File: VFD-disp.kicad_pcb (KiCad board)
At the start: 2 copper layers, 120.2 x 65.5 mm, 97 parts, among them J1 USB_C_Receptacle_USB2.0_14P, J2 Conn_02x04_Odd_Even, J3 Jack-DC, J4 Conn_02x04_Odd_Even, J5 Conn_02x04_Odd_Even, J6 Conn_02x04_Odd_Even, Q1 NMOS, Q3 NMOS, SW1 SW_SPST, U1 ESP32-C6-WROOM-1, U10 TXS0104EPW, U11 MAX811TEUS-T, U12 MCP4728, U2 FUSB302B01MPX, U3 LM1117DT-3.3, U4 MCP1416, U5 LM2576HVS-ADJ, U6 MAX1771xSA, U7 LM2576HVS-ADJ, U9 FM24C64B, Y1 Crystal

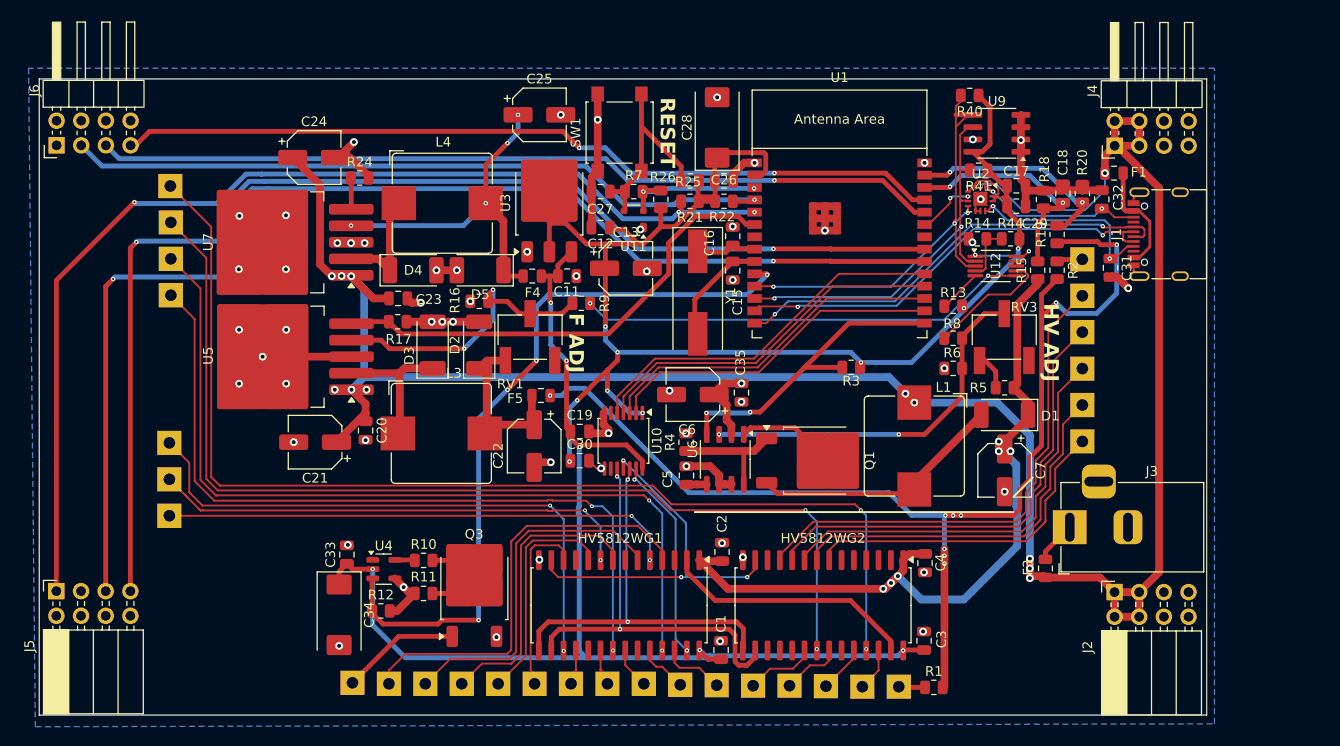
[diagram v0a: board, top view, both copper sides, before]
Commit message: We need to golf!
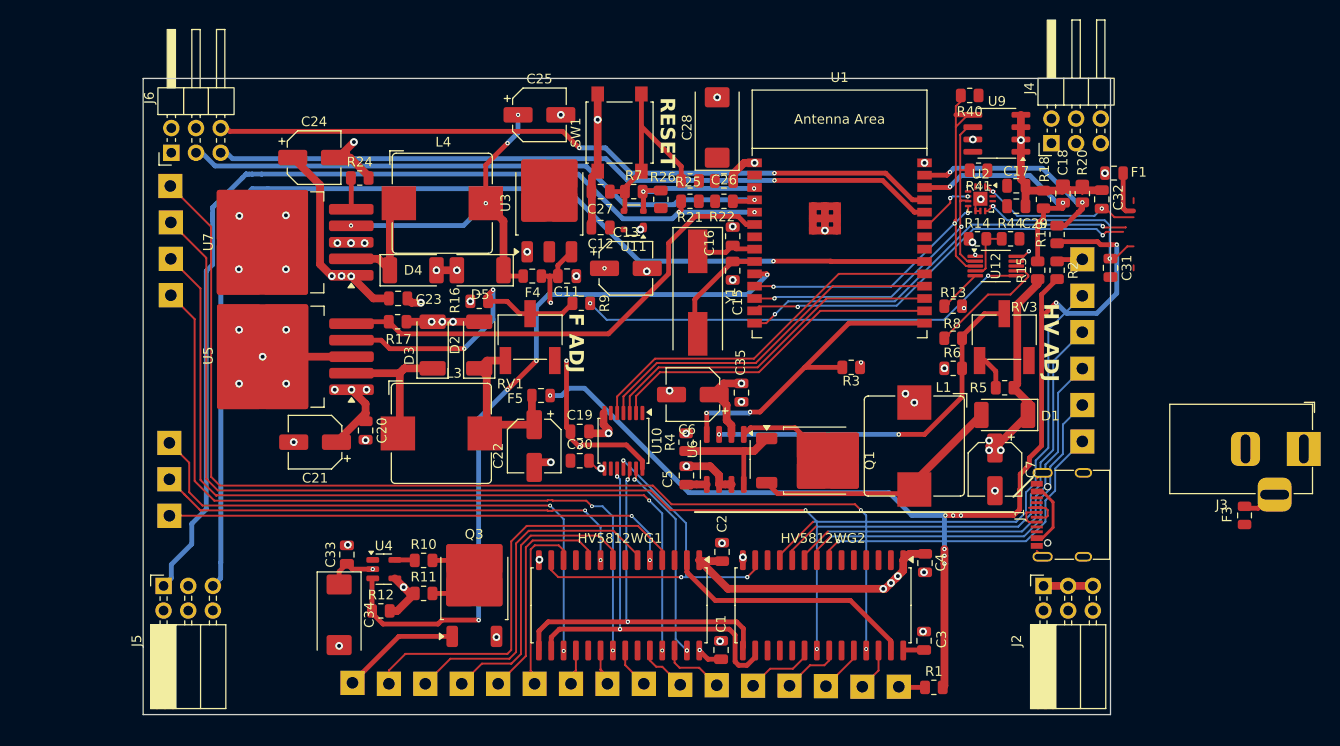
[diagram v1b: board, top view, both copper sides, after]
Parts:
- J2, J5: value Conn_02x04_Odd_Even -> Conn_02x03_Odd_Even; footprint Connector_PinSocket_2.54mm:PinSocket_2x04_P2.54mm_Horizontal -> Connector_PinSocket_2.54mm:PinSocket_2x03_P2.54mm_Horizontal
- J4, J6: value Conn_02x04_Odd_Even -> Conn_02x03_Odd_Even; footprint Connector_PinHeader_2.54mm:PinHeader_2x04_P2.54mm_Horizontal -> Connector_PinHeader_2.54mm:PinHeader_2x03_P2.54mm_Horizontal
- moved J1 30.6 mm to (134.8, 234.2)
- moved J3 25.4 mm to (158.6, 227.4), turned to 0 degrees
- moved F3 21.2 mm to (152.5, 234.2)
- moved J6 11.8 mm to (42.0, 196.9)
- moved J5 11.0 mm to (41.2, 241.5)
- moved J2 7.34 mm to (131.8, 241.5)
- moved J4 6.51 mm to (132.6, 195.9)
- moved C7 1.00 mm to (126.8, 229.5)
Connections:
- J2 pad 2: VBUS -> GND
- J2 pad 4: VBUS -> GND
- J2 pad 5: GND -> VBUS
- J4 pad 2: VBUS -> GND
- J4 pad 4: VBUS -> GND
- J4 pad 5: GND -> VBUS
- J5 pad 6: GND -> RX2
- J6 pad 6: GND -> TX1
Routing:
- net RX2: track 124.7 -> 0.00 mm, vias 2 -> 0
- net +3.3V: track 171.6 -> 65.8 mm, vias 10 -> 4
- net VBUS: track 243.7 -> 172.9 mm, vias 14 -> 11
- net +5V: track 127.9 -> 105.5 mm, vias 6 -> 5
- net GND: track 124.8 -> 107.7 mm, vias 59 -> 58
- net FORWARD_DETECT: track 74.4 -> 61.4 mm
- net RX1: track 87.1 -> 74.4 mm
- net Net-(Q3-G): track 17.0 -> 4.62 mm
- net TX2: track 126.4 -> 114.9 mm, vias 2 -> 1
- net Net-(Q1-G): track 18.7 -> 8.08 mm
- net TX1: track 85.5 -> 74.9 mm
- net BACKWARD_DETECT: track 111.9 -> 101.7 mm, vias 3 -> 2
- net Net-(D2-K): track 19.6 -> 15.4 mm
- net Net-(U1-GPIO1/ADC1_CH1/XTAL_32K_N): track 12.8 -> 10.1 mm
- net VPP: track 81.6 -> 79.7 mm
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- added copper zone on In2.Cu, net +3.3V
- added copper zone on In1.Cu, net GND
- removed copper zone on B.Cu, net GND
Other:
- board size 120.2 x 65.5 mm -> 99.6 x 65.5 mm
- copper layers 2 -> 4
